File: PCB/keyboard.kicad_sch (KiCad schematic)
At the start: 123 parts, among them SW1 SW_Push, SW10 SW_Push, SW11 SW_Push, SW12 SW_Push, SW13 SW_Push, SW14 SW_Push, SW15 SW_Push, SW16 SW_Push, SW17 SW_Push, SW18 SW_Push, SW19 SW_Push, SW2 SW_Push, SW20 SW_Push, SW21 SW_Push, SW22 SW_Push, SW23 SW_Push, SW24 SW_Push, SW25 SW_Push, SW26 SW_Push, SW27 SW_Push, SW28 SW_Push, SW29 SW_Push, SW3 SW_Push, SW30 SW_Push, SW31 SW_Push, SW32 SW_Push, SW33 SW_Push, SW34 SW_Push, SW35 SW_Push, SW36 SW_Push, SW37 SW_Push, SW38 SW_Push, SW39 SW_Push, SW4 SW_Push, SW40 SW_Push, SW41 SW_Push, SW42 SW_Push, SW43 SW_Push, SW44 SW_Push, SW45 SW_Push, SW46 SW_Push, SW47 SW_Push, SW48 SW_Push, SW49 SW_Push, SW5 SW_Push, SW50 SW_Push, SW51 SW_Push, SW52 SW_Push, SW53 SW_Push, SW54 SW_Push, SW55 SW_Push, SW56 SW_Push, SW57 SW_Push, SW58 SW_Push, SW59 SW_Push, SW6 SW_Push, SW60 SW_Push, SW61 SW_Push, SW7 SW_Push, SW8 SW_Push, SW9 SW_Push, U1 Pico

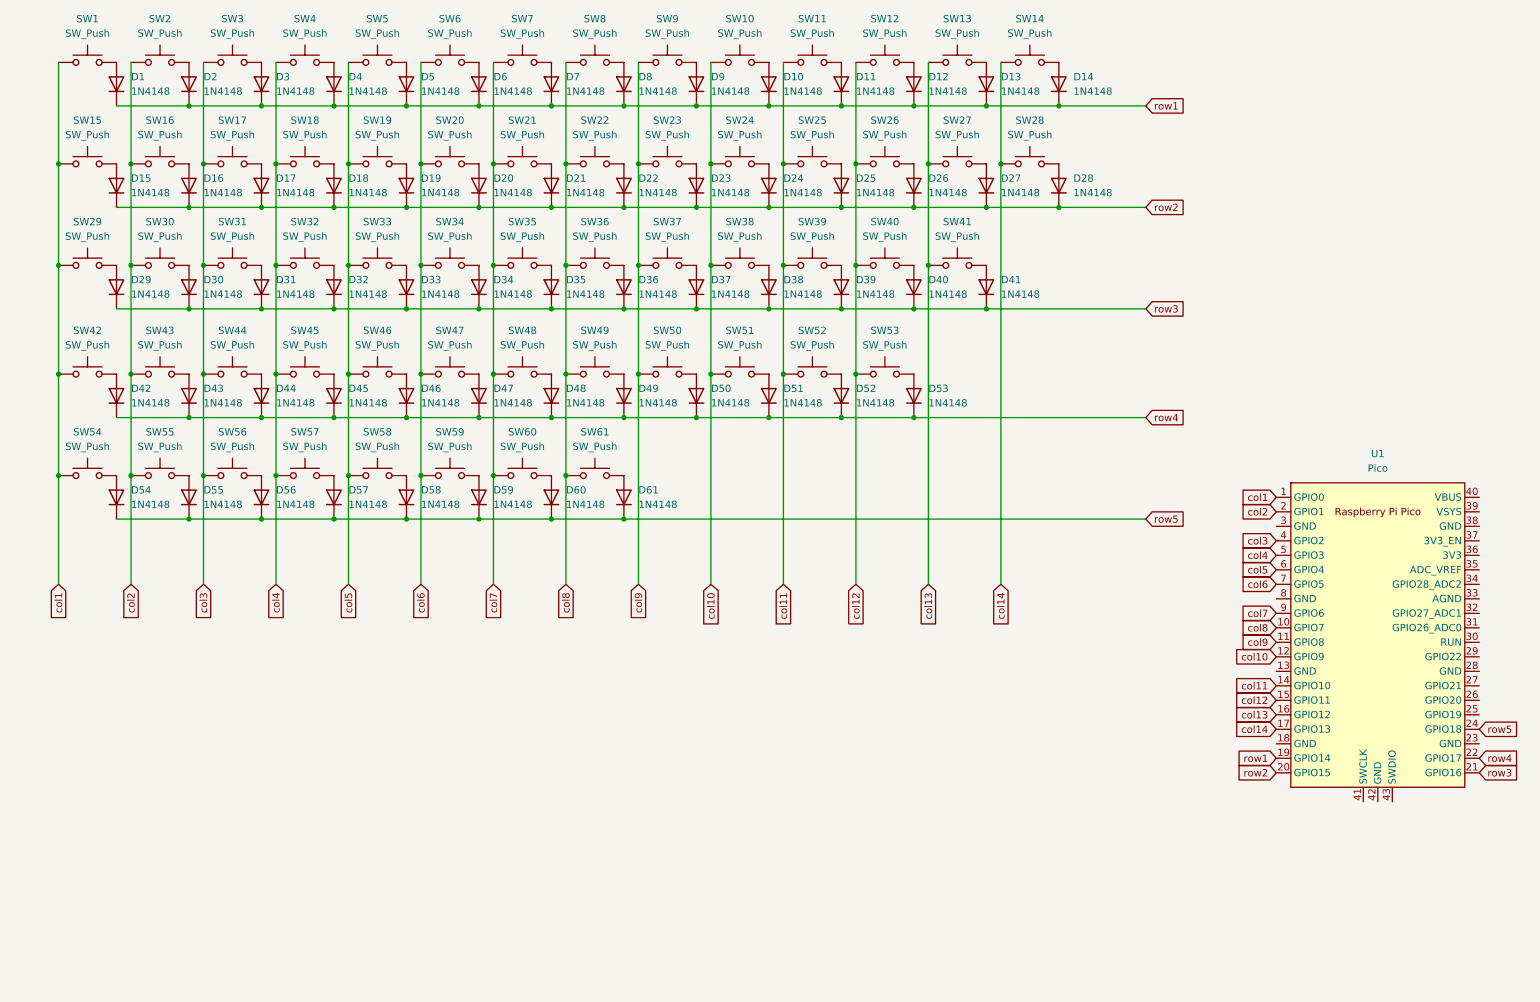
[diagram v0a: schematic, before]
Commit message: add PCB
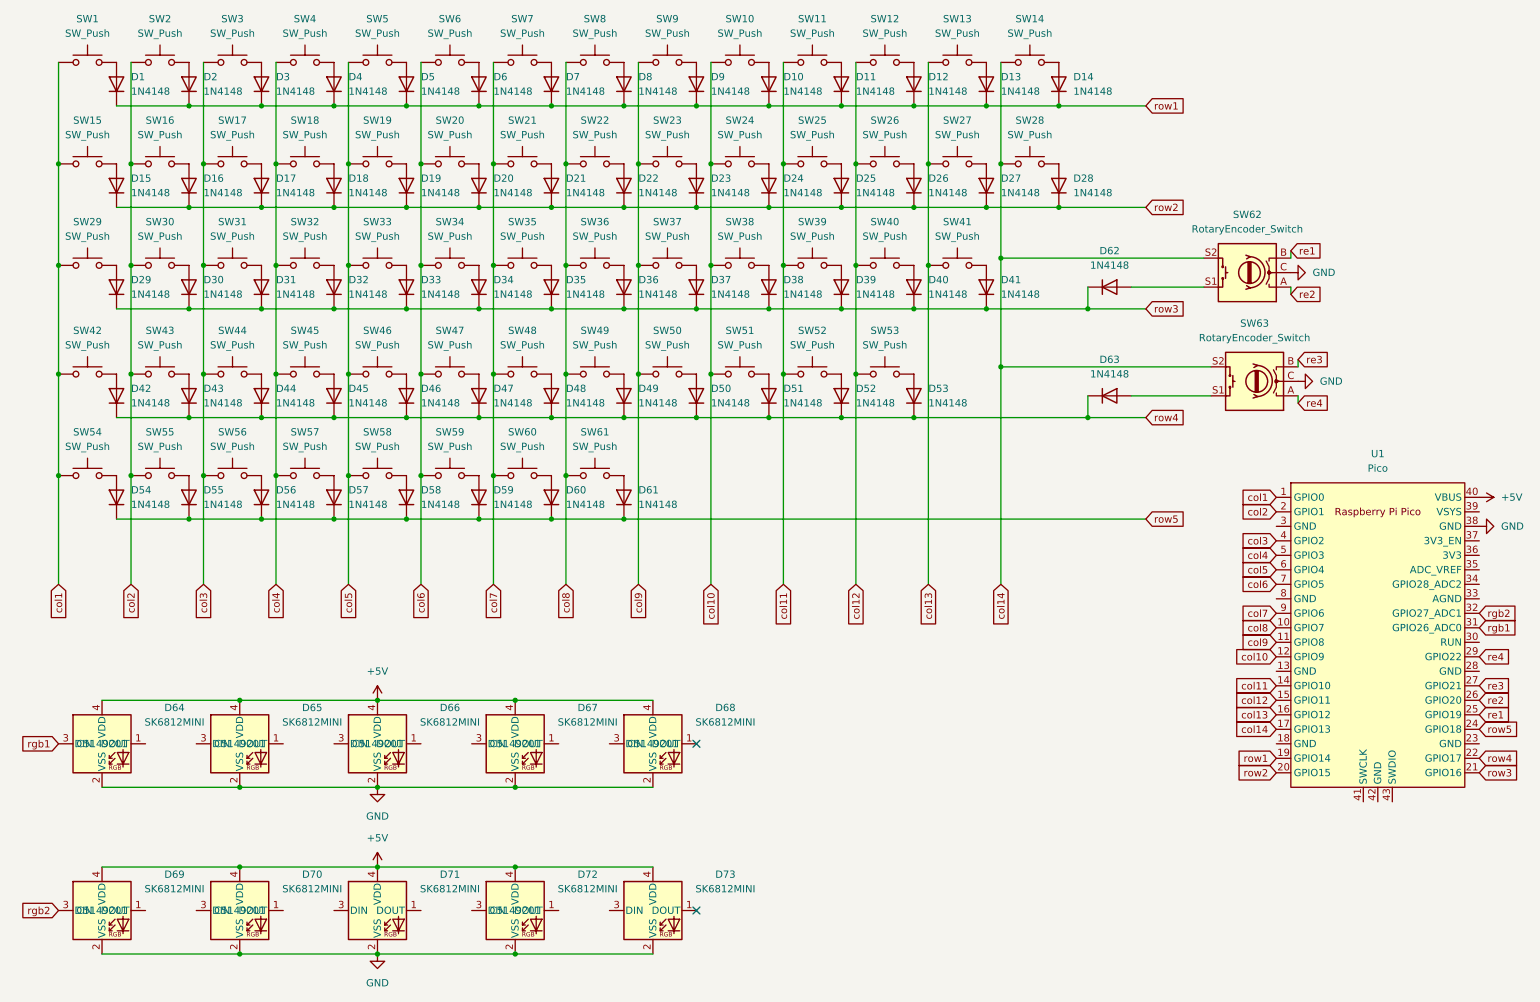
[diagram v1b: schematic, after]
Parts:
- added D62, D63: 1N4148, Diode_THT:D_DO-35_SOD27_P7.62mm_Horizontal, symbol Diode:1N4148
- added D64, D65, D66, D67, D68, D69, D70, D71, D72, D73: SK6812MINI, LED_SMD:LED_SK6812MINI_PLCC4_3.5x3.5mm_P1.75mm, symbol LED:SK6812MINI
- added SW62, SW63: RotaryEncoder_Switch, Rotary_Encoder:RotaryEncoder_Alps_EC11E-Switch_Vertical_H20mm_CircularMountingHoles, symbol Device:RotaryEncoder_Switch
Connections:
- net col14: now also SW62.S2, SW63.S2
- net row3: now also D62.1 (K)
- net row4: now also D63.1 (K)
- net re1: now reaches U1.25 (GPIO19)
- net re1: now also SW62.B
- net re2: now reaches U1.26 (GPIO20)
- net re2: now also SW62.A
- net re3: now reaches U1.27 (GPIO21)
- net re3: now also SW63.B
- net re4: now reaches U1.29 (GPIO22)
- net re4: now also SW63.A
- net rgb1: now reaches U1.31 (GPIO26_ADC0)
- net rgb1: now also D64.3 (DIN)
- net rgb2: now reaches U1.32 (GPIO27_ADC1)
- net rgb2: now also D69.3 (DIN)
- net GND: now reaches U1.38 (GND)
- net GND: now also D64.2 (VSS), D65.2 (VSS), D66.2 (VSS), D67.2 (VSS), D68.2 (VSS), D69.2 (VSS), D70.2 (VSS), D71.2 (VSS), D72.2 (VSS), D73.2 (VSS), SW62.C, SW63.C
- net +5V: now reaches U1.40 (VBUS)
- net +5V: now also D64.4 (VDD), D65.4 (VDD), D66.4 (VDD), D67.4 (VDD), D68.4 (VDD), D69.4 (VDD), D70.4 (VDD), D71.4 (VDD), D72.4 (VDD), D73.4 (VDD)
- new net: D62.2 (A), SW62.S1
- new net: D63.2 (A), SW63.S1
- no-connect marks 0 -> 2
